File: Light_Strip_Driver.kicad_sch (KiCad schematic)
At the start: 36 parts, among them J1 LED_S2, J10 BUCK3_IN, J11 BUCK3_OUT, J2 LED_S1, J3 DC_PWR, J4 FAN_PWR, J5 FAN_PWR, J6 BUCK1_IN, J7 BUCK1_OUT, J8 BUCK2_IN, J9 BUCK2_OUT, Q2 IRF4905, SW1 PWR_SW, SW10 PRE7, SW2 NEXT, SW3 PREV, SW4 PRE1, SW5 PRE2, SW6 PRE3, SW7 PRE4, SW8 PRE5, SW9 PRE6, U1 LS20-X

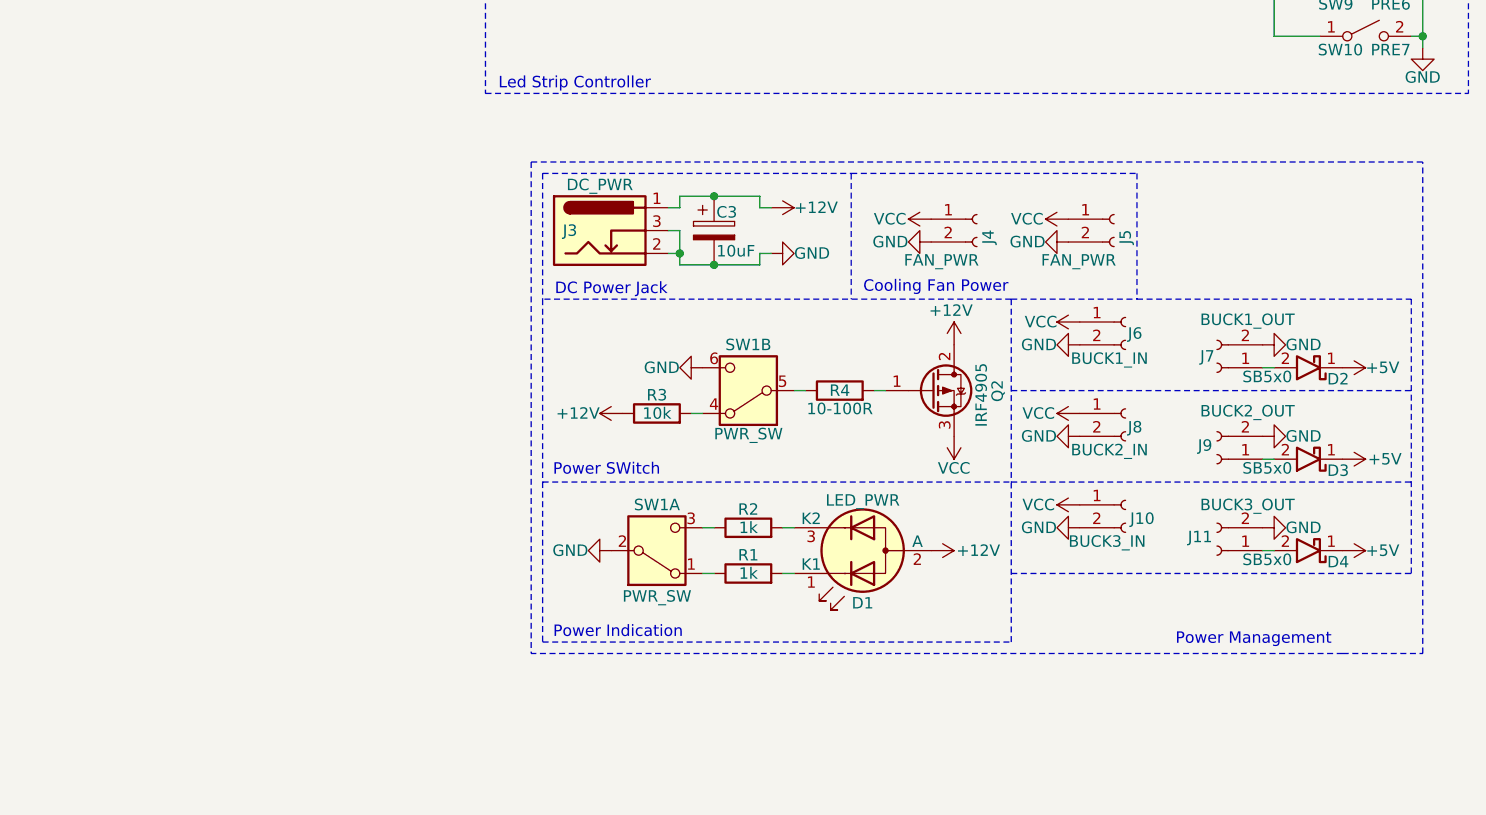
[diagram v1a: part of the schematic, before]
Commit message: finished pcb design
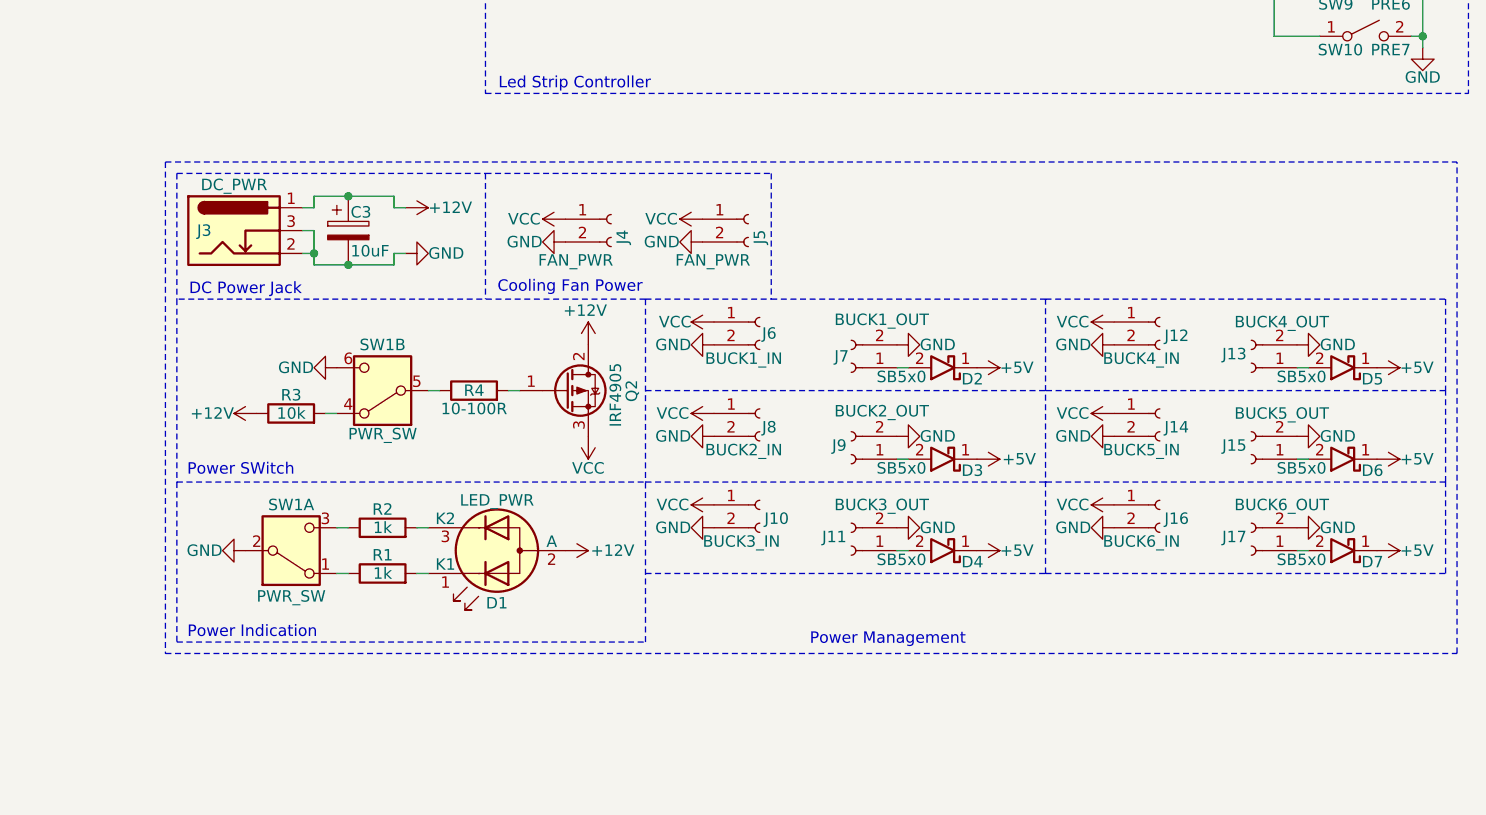
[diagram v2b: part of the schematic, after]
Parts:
- added D5, D6, D7: SB5x0, Diode_THT:D_DO-201AD_P12.70mm_Horizontal, symbol Custom:SB5x0
- added J12: BUCK4_IN, Connector_PinSocket_2.54mm:PinSocket_1x02_P2.54mm_Vertical, symbol Connector:Conn_01x02_Socket
- added J13: BUCK4_OUT, Connector_PinSocket_2.54mm:PinSocket_1x02_P2.54mm_Vertical, symbol Connector:Conn_01x02_Socket
- added J14: BUCK5_IN, Connector_PinSocket_2.54mm:PinSocket_1x02_P2.54mm_Vertical, symbol Connector:Conn_01x02_Socket
- added J15: BUCK5_OUT, Connector_PinSocket_2.54mm:PinSocket_1x02_P2.54mm_Vertical, symbol Connector:Conn_01x02_Socket
- added J16: BUCK6_IN, Connector_PinSocket_2.54mm:PinSocket_1x02_P2.54mm_Vertical, symbol Connector:Conn_01x02_Socket
- added J17: BUCK6_OUT, Connector_PinSocket_2.54mm:PinSocket_1x02_P2.54mm_Vertical, symbol Connector:Conn_01x02_Socket
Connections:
- net +5V: now also D5.1, D6.1, D7.1
- net GND: now also J12.2 (Pin_2), J13.2 (Pin_2), J14.2 (Pin_2), J15.2 (Pin_2), J16.2 (Pin_2), J17.2 (Pin_2)
- net VCC: now also J12.1 (Pin_1), J14.1 (Pin_1), J16.1 (Pin_1)
- new net: D7.2, J17.1 (Pin_1)
- new net: D6.2, J15.1 (Pin_1)
- new net: D5.2, J13.1 (Pin_1)
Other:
- moved on the sheet: C3, D1, D2, D3, D4, J10, J11, J3, J4, J5, J6, J7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
